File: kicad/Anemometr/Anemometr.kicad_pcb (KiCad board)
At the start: 2 copper layers, 44.9 x 45.2 mm, 164 parts, among them J10 +Z3, J11 -Z3, J12 +Z4, J13 -Z4, J14 SWD, J15 SWC, J16 Z4, J17 Z4, J18 1 TxD+, J19 2 TxD-, J2 Conn_01x01_Female, J20 3 RxD+, J21 4, J22 5, J23 6 RxD-, J24 7, J25 8, J26 Z4, J27 Z4, J28 Z4, J29 Z4, J3 RST, J30 Z4, J31 Z4, J32 Z4, J33 Z4, J34 Z4, J35 Z4, J4 TxD, J5 RxD, J6 +Z1, J7 -Z1, J8 +Z2, J9 -Z2, Q1 5N10, U1 TS5A3166DBVR, U10 MCP1700-3002E, U2 LMV7239, U3 TS5A3166DBVR, U4 TS5A3166DBVR, U5 STM32F103C8Tx, U6 TS5A3166DBVR, U7 LM2734Y, U8 MCP1700-5002E, U9 MCP1700-3002E, Y1 8MHz, Y2 25MHz

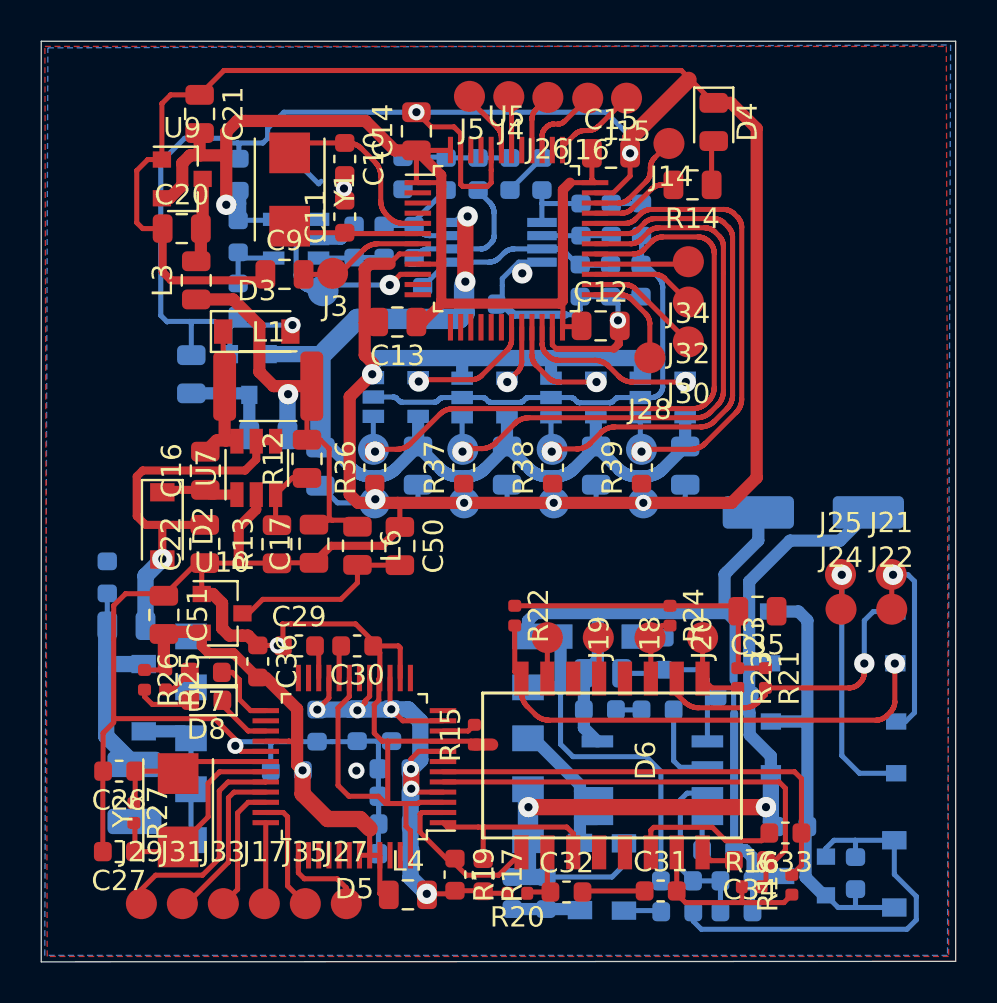
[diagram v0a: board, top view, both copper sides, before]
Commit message: изменено:      kicad/Anemometr/Anemometr.kicad_pcb 	изменено:      kicad/Anemometr/Anemometr.kicad_pcb-bak 	изменено:      kicad/Anemometr/Anemometr.sch 	изменено:      kicad/Anemometr/Anemometr.sch-bak 	изменено:      kicad/Anemometr/fp-info-cache
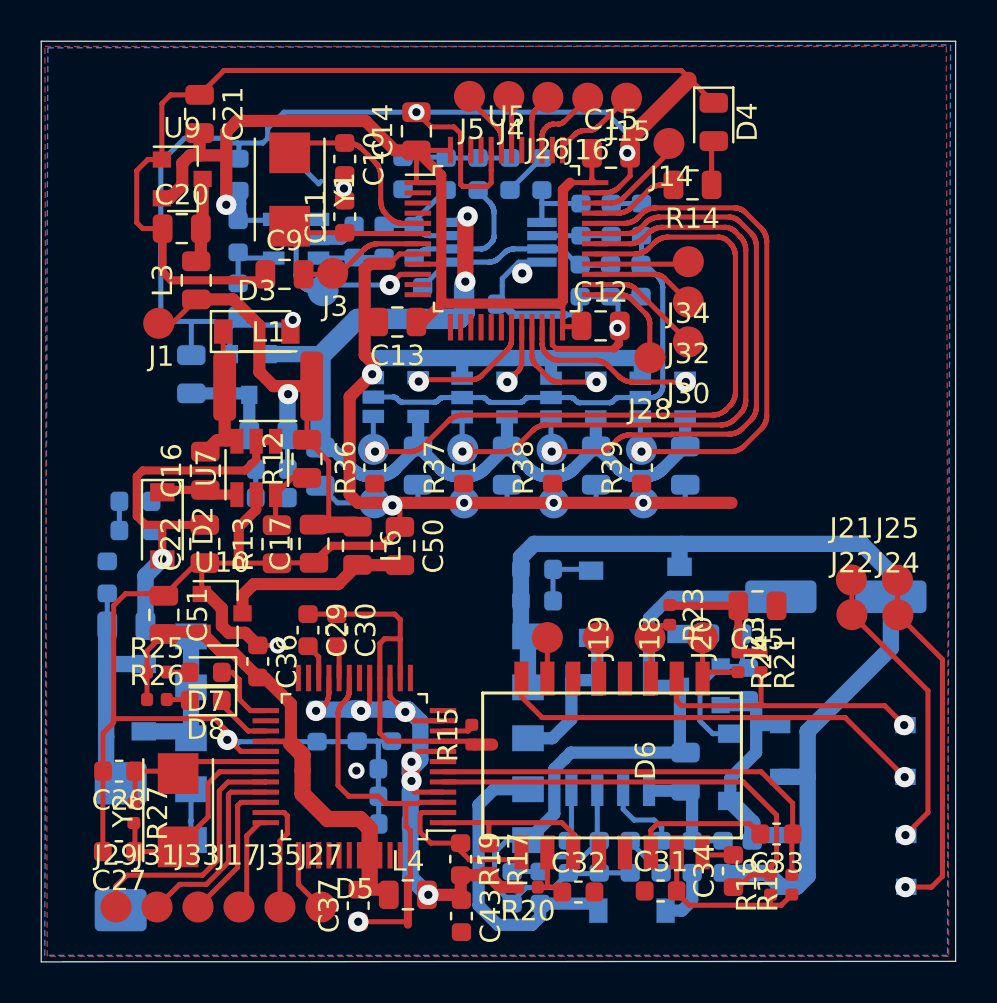
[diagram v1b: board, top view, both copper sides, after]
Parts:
- removed R22: 75R, Resistor_SMD:R_0402_1005Metric
- added D18: LED, LED_SMD:LED_0603_1608Metric, B.Cu at (23.5, 82.2)
- added D19: LED, LED_SMD:LED_0603_1608Metric, B.Cu at (30.2, 82.0)
- added J1: +5.5v, My-library:SMD-CONN, F.Cu at (24.6, 73.4)
- added R43: 4.7k, Resistor_SMD:R_0603_1608Metric, B.Cu at (23.5, 83.6)
- added R44: 2k, Resistor_SMD:R_0603_1608Metric, B.Cu at (30.2, 80.6)
- C37, C43: moved to F.Cu
- C49: value 20uF -> 220uF; footprint Capacitor_SMD:C_1210_3225Metric -> Capacitor_Tantalum_SMD:CP_EIA-7343-15_Kemet-W
- moved C48 15.9 mm to (43.2, 85.5), turned to 0 degrees
- moved R34 14.4 mm to (43.2, 87.1), turned to 0 degrees
- moved D16 13.8 mm to (50.2, 87.0)
- moved R40 13.8 mm to (52.5, 88.7)
- moved D11 13.6 mm to (47.9, 102.3)
- moved D13 13.4 mm to (45.9, 87.2), turned to 270 degrees
- moved R30 11.0 mm to (42.0, 101.1), turned to 270 degrees
- moved Q1 10.7 mm to (51.2, 91.2)
- moved R42 10.7 mm to (53.6, 91.1)
- moved R31 10.1 mm to (50.8, 99.6), turned to 90 degrees
- moved D17 9.60 mm to (52.7, 95.2), turned to 90 degrees
- moved R28 7.89 mm to (52.3, 99.6), turned to 90 degrees
- moved C37 7.49 mm to (34.4, 102.0), turned to 90 degrees
- moved C47 7.37 mm to (47.8, 99.6), turned to 270 degrees
- moved R33 7.36 mm to (44.7, 99.6), turned to 270 degrees
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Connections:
- D17 pad 1: Net-(D17-Pad1) -> Net-(D10-Pad4)
- D17 pad 2: Net-(D10-Pad4) -> Net-(D17-Pad2)
- Q1 pad 1: Net-(D17-Pad1) -> Net-(D17-Pad2)
- R23 pad 2: Net-(D6-Pad9) -> Net-(D6-Pad11)
- R24 pad 2: Net-(D6-Pad11) -> Net-(D6-Pad9)
- R40 pad 1: Net-(D17-Pad1) -> Net-(D17-Pad2)
- R42 pad 1: Net-(D17-Pad1) -> Net-(D17-Pad2)
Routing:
- net GND: track 326.5 -> 303.5 mm, vias 14 -> 15
- net Net-(D17-Pad1): track 20.9 -> 0.00 mm
- net Net-(D10-Pad4): track 22.4 -> 12.0 mm
- net Net-(C35-Pad2): track 15.2 -> 6.60 mm
- net Net-(D17-Pad2): track 0.00 -> 8.02 mm
- net Net-(C45-Pad1): track 43.7 -> 49.3 mm, vias 2 -> 0
- net Net-(D10-Pad1): track 10.4 -> 14.5 mm
- net Net-(D10-Pad2): track 13.6 -> 17.5 mm
- net Net-(C17-Pad2): track 21.2 -> 24.7 mm
- net Net-(D6-Pad15): track 24.8 -> 21.3 mm
- net Net-(C45-Pad2): track 40.3 -> 37.1 mm
- net Net-(D11-Pad2): track 17.8 -> 14.9 mm
- net Net-(J12-Pad1): track 24.0 -> 26.7 mm
- net Net-(J10-Pad1): track 26.9 -> 29.4 mm
- net Net-(J8-Pad1): track 29.8 -> 32.3 mm
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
